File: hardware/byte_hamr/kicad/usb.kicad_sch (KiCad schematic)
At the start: 7 parts, among them J4 CONN_02X03, U1 LFE5U-85F-8BG381I, U6 FT231XQ

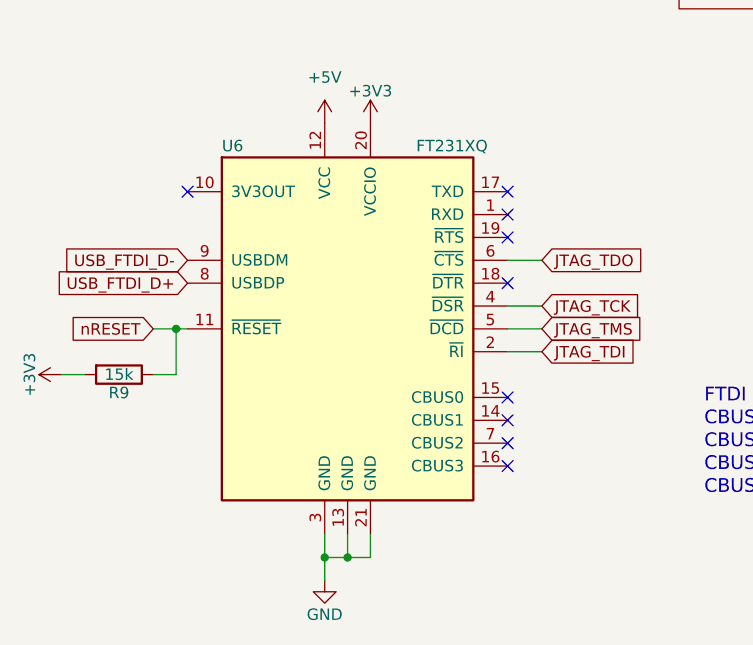
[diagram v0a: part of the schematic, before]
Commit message: Fabrication Feedback
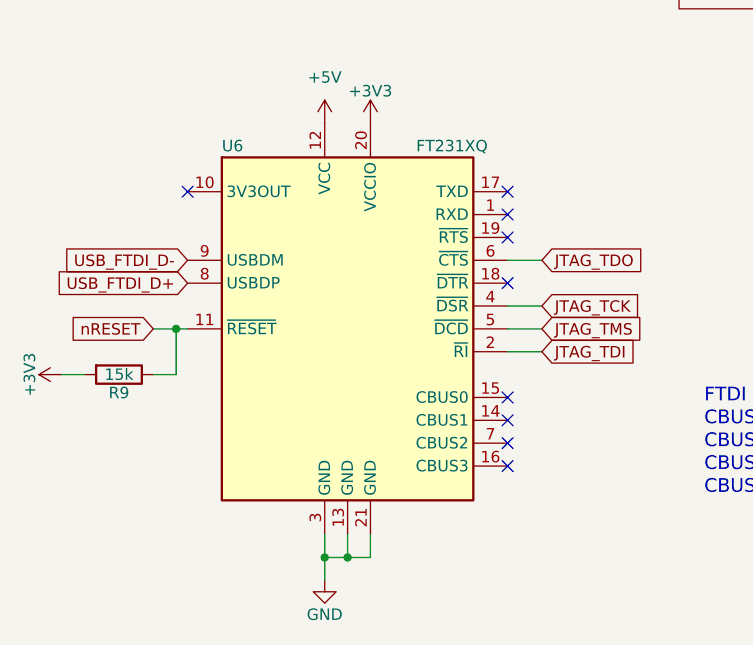
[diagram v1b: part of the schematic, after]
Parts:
- J4: Side T -> (none)
- R49: Digikey 311-27.0HRCT-ND -> (none); Koncar FR008 -> (none); LCSC C325726 -> (none); MNF1_URL www.yageo.com -> (none); MPN AC0603JR-0727RL -> RC0603FR-0727RL; Mouser 603-AC0603JR-0727RL -> (none); Newark 08AH8595 -> (none)
- R50: MNF1_URL www.yageo.com -> (none); MPN AC0603JR-0727RL -> RC0603FR-0727RL
- R9: Digikey YAG3569CT-ND -> (none); Koncar FR005 -> (none); LCSC C217750 -> (none); MNF1_URL www.yageo.com -> (none); Mouse_r1 603-RC0603FR-0715KL -> (none); Mouse_r2 603-RC0603FR-1015KL -> (none); Mouse_r3 603-RC0603FR-1315KL -> (none); Mouser 603-AC0603FR-1015KL -> (none); Newark 94X1443 -> (none); price1500_Mouser 8.4$ -> (none)
- U6: footprint ft231x:FT231X-QFN-20-1EP_4x4mm_P0.5mm_EP2x2mm -> Package_DFN_QFN:QFN-20-1EP_4x4mm_P0.5mm_EP2.5x2.5mm; symbol ftdi:FT231XQ -> Interface_USB:FT231XQ; Digikey 768-1128-1-ND -> (none); Dikike_y2 768-1155-ND -> (none); Koncar FU002 -> (none); LCSC C132159 -> (none); MNF1_URL www.ftdichip.com -> (none); MPN FT231XQ -> FT231XQ-R; Mouse_r2 895-FT231XQ-T -> (none); Mouser 895-FT231XQ-R -> (none); Newark 83T7088 -> (none); RS 7570032 -> (none); price100_RS 1.86$ -> (none)
- US1: Datasheet2 https://www.molex.com/pdm_docs/sd/473460001_sd.pdf -> (none); Digikey 609-4613-1-ND -> (none); Digikey2 WM17141CT-ND -> (none); FreelanceElec 10118192-0001LF -> (none); Koncar FU010 -> (none); LCSC C132564 -> (none); MFG1 FCI -> (none); MFG2 Molex -> (none); MNF1_URL www.fciconnect.com -> (none); MNF2_URL www.molex.com -> (none); MPN2 47346-0001 -> (none); Mouse_r1 538-47346-0001 -> (none); Mouse_r2 490-UJ2-MIBH-G-SMTTR -> (none); Mouser 649-10118192-0001LF -> (none); Newark 47M0505 -> (none); Side T -> (none); price200_FreelanceElec 0.12487$ -> (none)

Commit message: FTDI Update
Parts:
- U6: footprint Package_DFN_QFN:QFN-20-1EP_4x4mm_P0.5mm_EP2.5x2.5mm -> ft231x:FT231X-QFN-20-1EP_4x4mm_P0.5mm_EP2x2mm
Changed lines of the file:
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@@
 			)
 		)
-		(property "Footprint" "Package_DFN_QFN:QFN-20-1EP_4x4mm_P0.5mm_EP2.5x2.5mm"
+		(property "Footprint" "ft231x:FT231X-QFN-20-1EP_4x4mm_P0.5mm_EP2x2mm"
 			(at 101.6 120.65 0)
 			(effects
